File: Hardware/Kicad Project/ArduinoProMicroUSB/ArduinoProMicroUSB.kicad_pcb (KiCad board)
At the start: 4 copper layers, 31.1 x 26 mm, 51 parts, among them J3 Display FPC, Q1 MMBT3904, U1 RV-3028-C7, U2 MIC5219, U3 USB-AB, U5 ATMEGA32U4QFN, Y1 16MHz

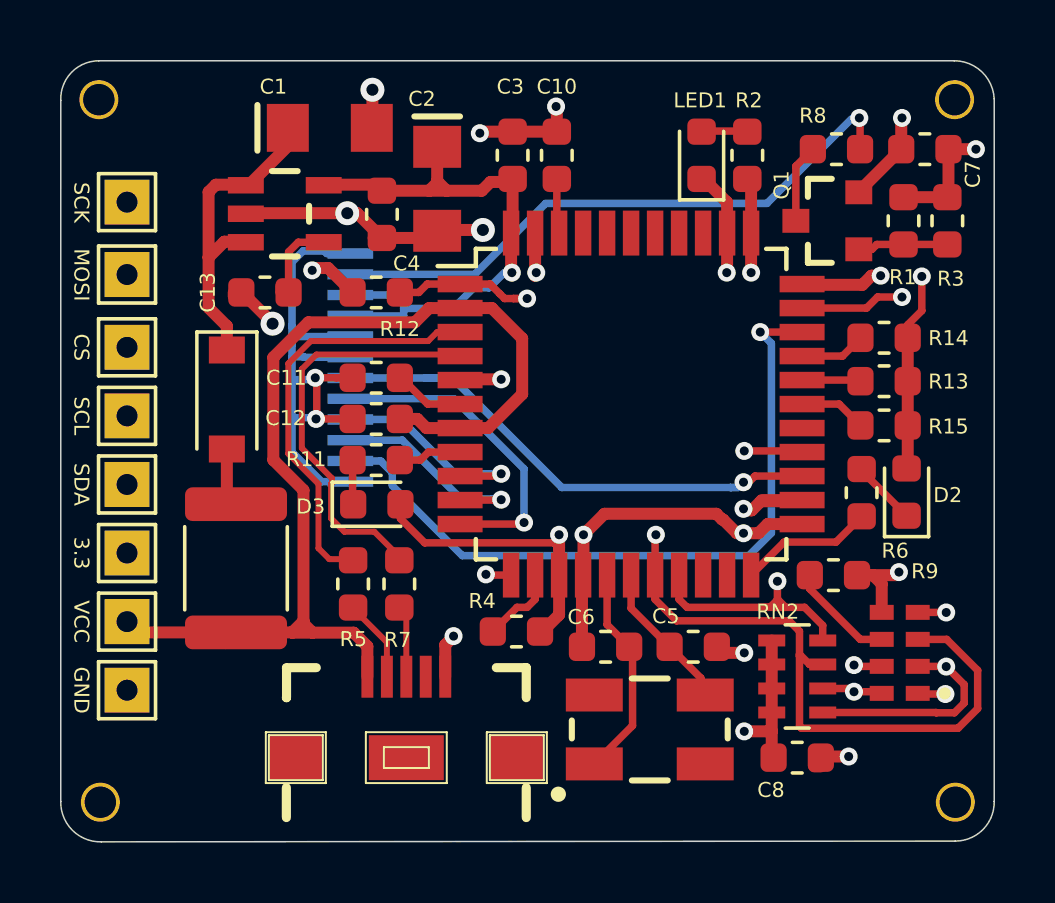
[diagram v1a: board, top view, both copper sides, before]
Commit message: rev 0.3
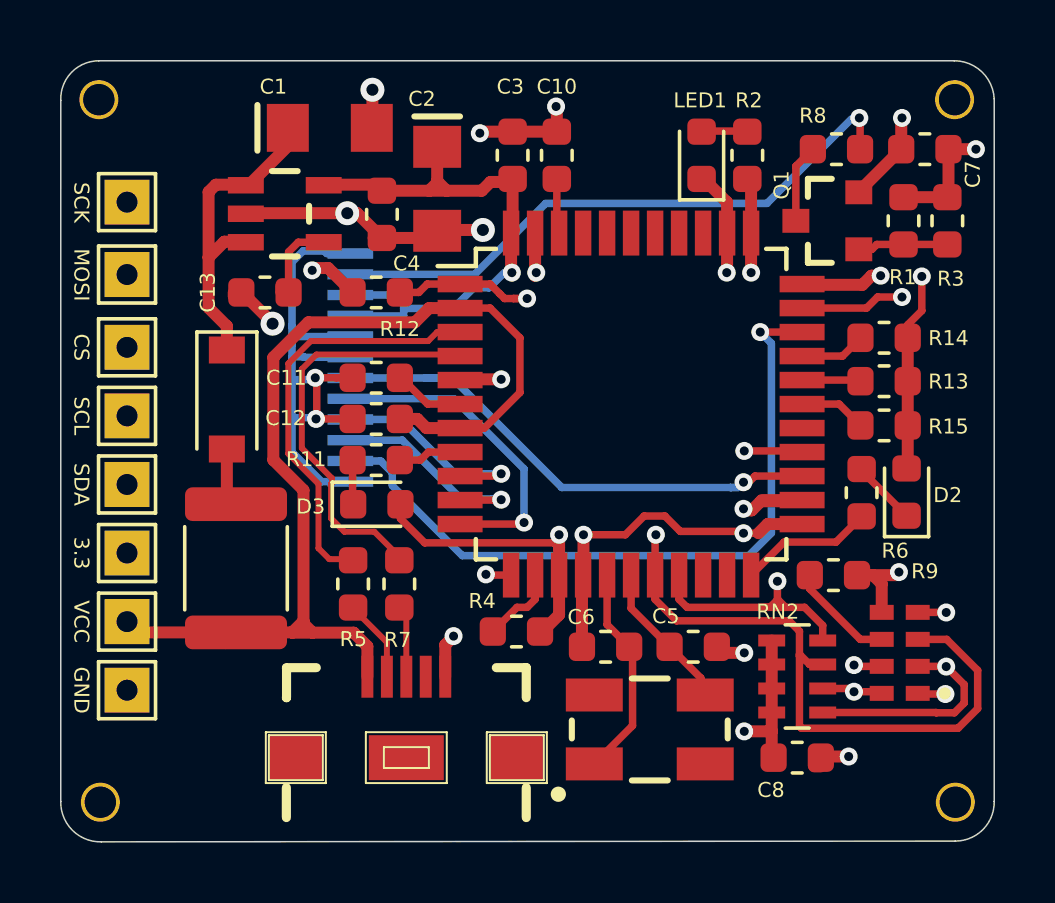
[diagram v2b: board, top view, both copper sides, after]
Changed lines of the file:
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@@
     (35 F.Paste user hide)
     (36 B.SilkS user hide)
-    (37 F.SilkS user)
+    (37 F.SilkS user hide)
     (38 B.Mask user hide)
     (39 F.Mask user hide)
@@
   )
   (setup
-    (last_trace_width 0.4)
+    (last_trace_width 0.25)
     (user_trace_width 0.15)
     (user_trace_width 0.2)
@@
       (effects (font (size 1 1) (thickness 0.15)))
     )
-    (fp_text user %R (at 8.001 -1.7145) (layer F.Fab)
-      (effects (font (size 1 1) (thickness 0.15)))
-    )
     (fp_circle (center 0 0) (end 1.05 0) (layer Cmts.User) (width 0.15))
     (fp_circle (center 0 0) (end 1.3 0) (layer F.CrtYd) (width 0.05))
+    (fp_text user %R (at 8.001 -1.7145) (layer F.Fab)
+      (effects (font (size 1 1) (thickness 0.15)))
+    )
     (pad "" np_thru_hole circle (at 0 0) (size 1.3 1.3) (drill 1.05) (layers *.Cu *.Mask))
   )
@@
       (effects (font (size 1 1) (thickness 0.15)))
     )
+    (fp_line (start 1.48 0.73) (end -1.48 0.73) (layer F.CrtYd) (width 0.05))
+    (fp_line (start 1.48 -0.73) (end 1.48 0.73) (layer F.CrtYd) (width 0.05))
+    (fp_line (start -1.48 -0.73) (end 1.48 -0.73) (layer F.CrtYd) (width 0.05))
+    (fp_line (start -1.48 0.73) (end -1.48 -0.73) (layer F.CrtYd) (width 0.05))
+    (fp_line (start -0.162779 0.51) (end 0.162779 0.51) (layer F.SilkS) (width 0.12))
+    (fp_line (start -0.162779 -0.51) (end 0.162779 -0.51) (layer F.SilkS) (width 0.12))
+    (fp_line (start 0.8 0.4) (end -0.8 0.4) (layer F.Fab) (width 0.1))
+    (fp_line (start 0.8 -0.4) (end 0.8 0.4) (layer F.Fab) (width 0.1))
+    (fp_line (start -0.8 -0.4) (end 0.8 -0.4) (layer F.Fab) (width 0.1))
+    (fp_line (start -0.8 0.4) (end -0.8 -0.4) (layer F.Fab) (width 0.1))
     (fp_text user %R (at 0 0 90) (layer F.Fab)
       (effects (font (size 0.4 0.4) (thickness 0.06)))
     )
-    (fp_line (start 1.48 0.73) (end -1.48 0.73) (layer F.CrtYd) (width 0.05))
-    (fp_line (start 1.48 -0.73) (end 1.48 0.73) (layer F.CrtYd) (width 0.05))
-    (fp_line (start -1.48 -0.73) (end 1.48 -0.73) (layer F.CrtYd) (width 0.05))
-    (fp_line (start -1.48 0.73) (end -1.48 -0.73) (layer F.CrtYd) (width 0.05))
-    (fp_line (start -0.162779 0.51) (end 0.162779 0.51) (layer F.SilkS) (width 0.12))
-    (fp_line (start -0.162779 -0.51) (end 0.162779 -0.51) (layer F.SilkS) (width 0.12))
-    (fp_line (start 0.8 0.4) (end -0.8 0.4) (layer F.Fab) (width 0.1))
-    (fp_line (start 0.8 -0.4) (end 0.8 0.4) (layer F.Fab) (width 0.1))
-    (fp_line (start -0.8 -0.4) (end 0.8 -0.4) (layer F.Fab) (width 0.1))
-    (fp_line (start -0.8 0.4) (end -0.8 -0.4) (layer F.Fab) (width 0.1))
     (pad 1 smd roundrect (at -0.7875 0 90) (size 0.875 0.95) (layers F.Cu F.Paste F.Mask) (roundrect_rratio 0.25)
       (net 17 "Net-(Q1-Pad1)"))
@@
   (segment (start 149.7486 90.17) (end 150.0539 89.8647) (width 0.4) (layer F.Cu) (net 2))
   (segment (start 150.0539 89.8647) (end 151.2039 89.8647) (width 0.4) (layer F.Cu) (net 2))
-  (segment (start 149.098 90.17) (end 149.7486 90.17) (width 0.4) (layer F.Cu) (net 2))
   (via (at 143.9164 90.2208) (size 0.6) (drill 0.3) (layers F.Cu B.Cu) (net 2))
   (segment (start 141.4781 76.835) (end 141.5288 76.8857) (width 0.4) (layer F.Cu) (net 2))
@@
   (segment (start 148.5647 94.1578) (end 148.3615 93.9546) (width 0.4) (layer F.Cu) (net 2))
   (segment (start 149.2758 94.1578) (end 148.5647 94.1578) (width 0.4) (layer F.Cu) (net 2))
-  (segment (start 143.9164 90.2208) (end 144.616401 89.520799) (width 0.4) (layer F.Cu) (net 2))
-  (segment (start 148.569998 89.7128) (end 149.027198 90.17) (width 0.4) (layer F.Cu) (net 2))
-  (segment (start 144.616401 89.520799) (end 148.347199 89.520799) (width 0.4) (layer F.Cu) (net 2))
-  (segment (start 148.347199 89.520799) (end 148.5392 89.7128) (width 0.4) (layer F.Cu) (net 2))
-  (segment (start 149.027198 90.17) (end 149.2504 90.17) (width 0.4) (layer F.Cu) (net 2))
-  (segment (start 148.5392 89.7128) (end 148.569998 89.7128) (width 0.4) (layer F.Cu) (net 2))
+  (segment (start 143.9164 90.2208) (end 145.3134 90.2208) (width 0.25) (layer F.Cu) (net 2))
+  (segment (start 146.629401 89.595799) (end 147.1422 90.108598) (width 0.25) (layer F.Cu) (net 2))
+  (segment (start 145.3134 90.2208) (end 145.938401 89.595799) (width 0.25) (layer F.Cu) (net 2))
+  (segment (start 145.938401 89.595799) (end 146.629401 89.595799) (width 0.25) (layer F.Cu) (net 2))
+  (segment (start 149.188998 90.108598) (end 149.2504 90.17) (width 0.25) (layer F.Cu) (net 2))
+  (segment (start 147.1422 90.108598) (end 149.188998 90.108598) (width 0.25) (layer F.Cu) (net 2))
+  (segment (start 149.2504 90.17) (end 149.7486 90.17) (width 0.25) (layer F.Cu) (net 2))
   (segment (start 146.684494 93.9546) (end 146.7865 93.9546) (width 0.25) (layer F.Cu) (net 3) (status 30))
   (segment (start 145.5039 92.672) (end 145.5039 91.5647) (width 0.25) (layer F.Cu) (net 3) (status 20))
@@
   (segment (start 134.88611 93.48411) (end 136.25771 93.48411) (width 0.4) (layer F.Cu) (net 7))
   (segment (start 139.804 86.6648) (end 139.8039 86.6647) (width 0.4) (layer F.Cu) (net 7))
-  (segment (start 140.861424 82.6647) (end 139.8039 82.6647) (width 0.4) (layer F.Cu) (net 7))
-  (segment (start 141.873201 83.676477) (end 140.861424 82.6647) (width 0.4) (layer F.Cu) (net 7))
-  (segment (start 140.7415 86.6647) (end 141.873201 85.532999) (width 0.4) (layer F.Cu) (net 7))
-  (segment (start 141.873201 85.532999) (end 141.873201 83.676477) (width 0.4) (layer F.Cu) (net 7))
-  (segment (start 139.8039 86.6647) (end 140.7415 86.6647) (width 0.4) (layer F.Cu) (net 7))
+  (segment (start 140.613902 86.6647) (end 139.8039 86.6647) (width 0.25) (layer F.Cu) (net 7))
+  (segment (start 141.798201 85.480401) (end 140.613902 86.6647) (width 0.25) (layer F.Cu) (net 7))
+  (segment (start 141.798201 83.659001) (end 141.798201 85.480401) (width 0.25) (layer F.Cu) (net 7))
+  (segment (start 140.8039 82.6647) (end 141.798201 83.659001) (width 0.25) (layer F.Cu) (net 7))
+  (segment (start 139.8039 82.6647) (end 140.8039 82.6647) (width 0.25) (layer F.Cu) (net 7))
   (segment (start 133.7819 82.1309) (end 133.8707 82.1309) (width 0.25) (layer F.Cu) (net 8))
   (segment (start 133.7692 82.1563) (end 133.7692 81.9276) (width 0.25) (layer F.Cu) (net 8))
